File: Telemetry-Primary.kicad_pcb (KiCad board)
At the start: 2 copper layers, 94.5 x 82 mm, 148 parts, among them J1 CAN_LogicAnalyzer, J10 SMAConn, J11 USB_B_Micro, J12 CAN_In, J13 CAN_Out, J2 IMU_LogicAnalyzer, J3 GPS_LogicAnalyzer, J5 SDCard_LogicAnalyzer, J6 SWD, J7 PowerConn, J8 RJ45_Abracon_ARJP11A-MASA-B-A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, J9 Micro_SD_Card_Det, SW1 Reset, SW2 RTCC_BattCheck, SW3 GPS_BattCheck, U1 STM32F429ZITx, U10 ADM3055E, U11 CDSOT23-T24CAN, U2 RI3-1205S, U3 NCP1117-3.3_SOT223, U4 LAN8742A-CZ-TR, U5 USBLC6-4SC6, U7 MTK3339, U8 BNO055, U9 CP2102N-A01-GQFN24, Y1 8M, Y2 25M, Y3 32.768k

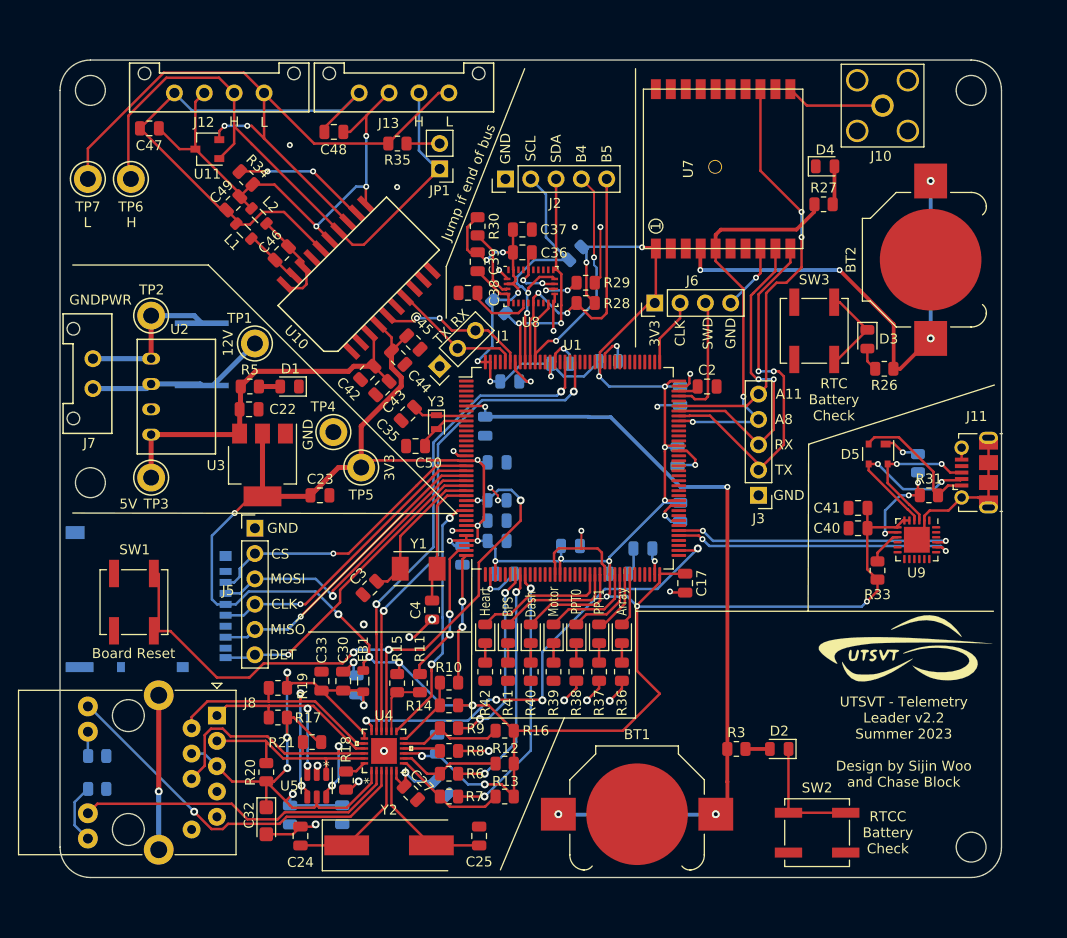
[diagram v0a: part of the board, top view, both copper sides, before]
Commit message: bom, gerbers, edge cuts, footprint verification
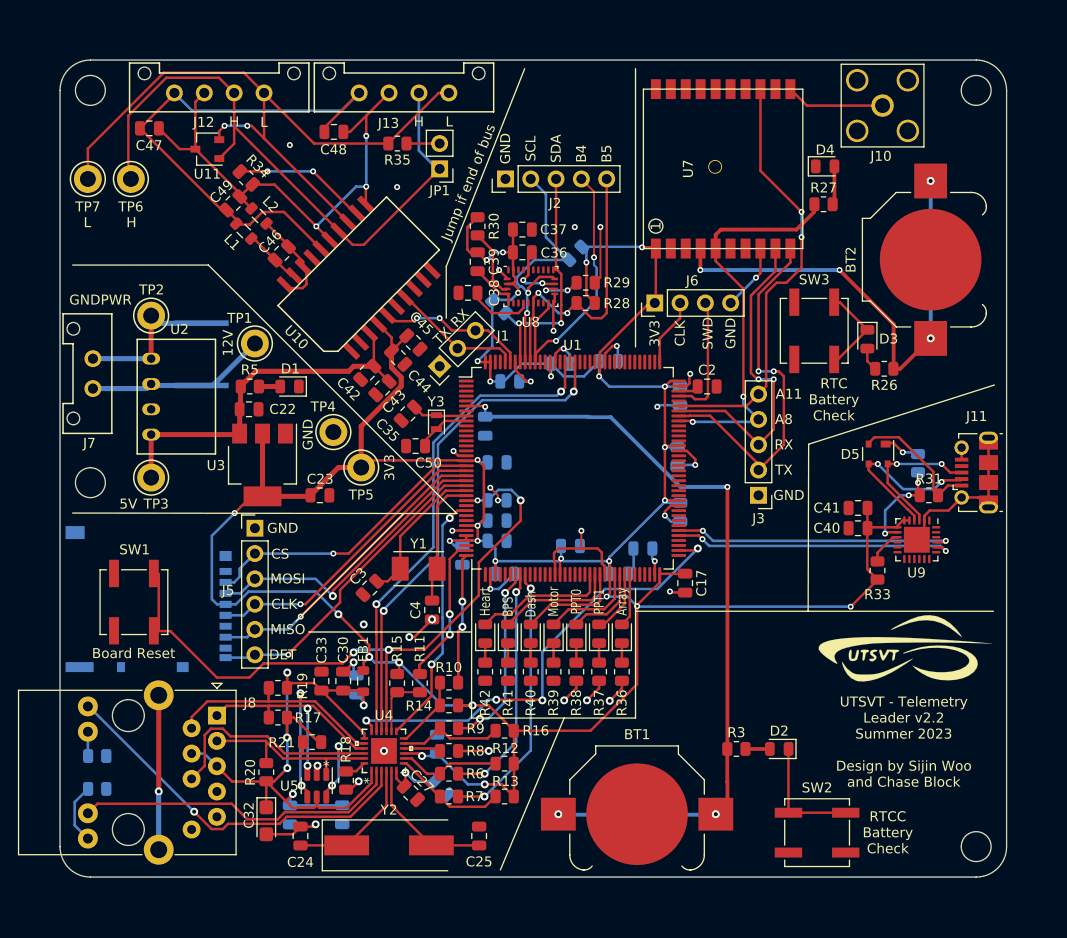
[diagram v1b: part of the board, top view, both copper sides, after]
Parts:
- moved H4 0.51 mm to (163.1, 123.9)
- moved H3 0.51 mm to (163.1, 48.0)
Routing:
- net +3.3V: track 354.2 -> 349.8 mm
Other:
- board size 94.5 x 82 mm -> 95 x 82 mm
